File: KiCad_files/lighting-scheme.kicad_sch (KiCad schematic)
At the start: 11 parts, among them J1 Conn_01x03

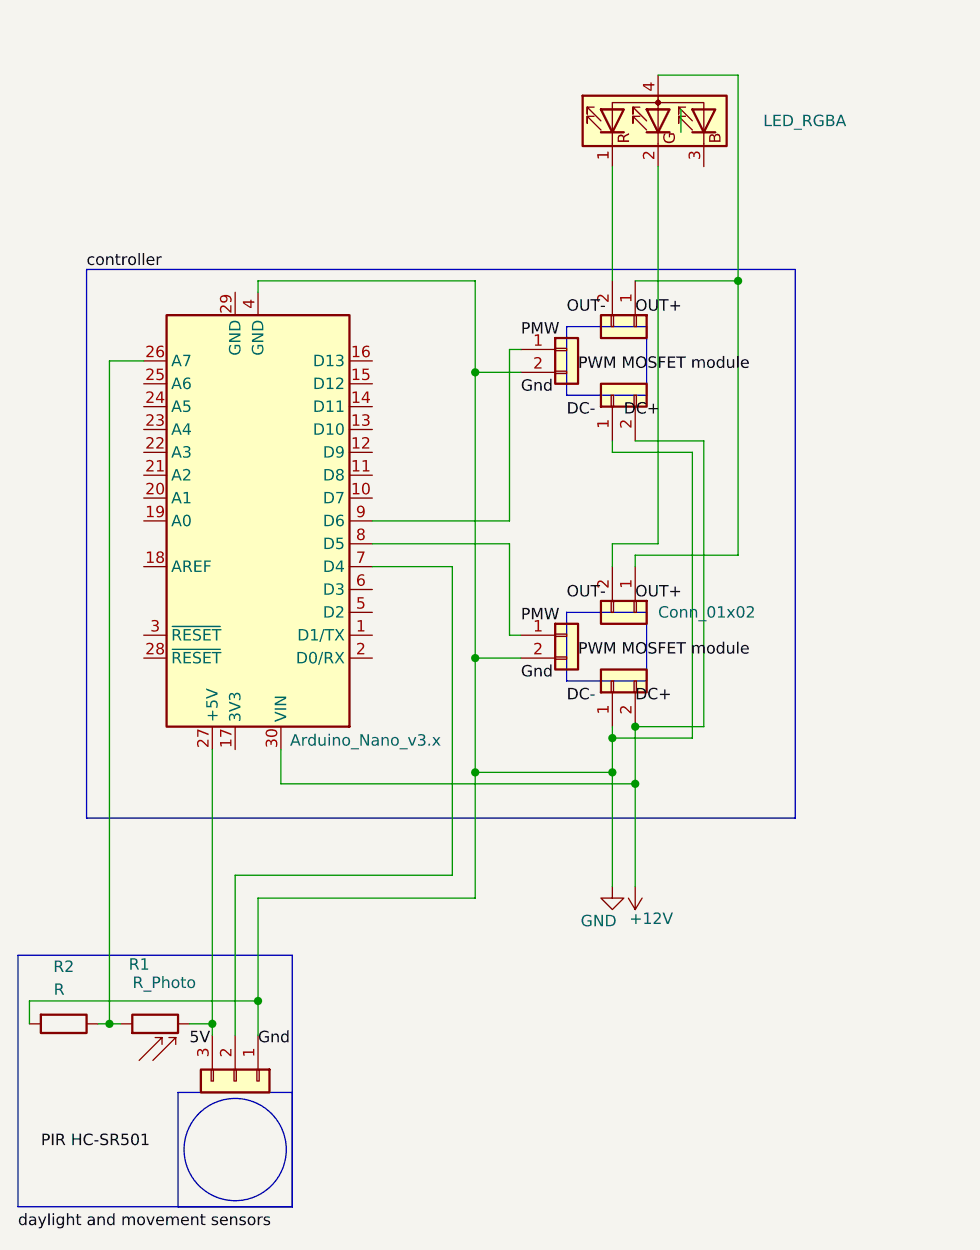
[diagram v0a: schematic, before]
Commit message: aktuallizacja folder z kicad 2
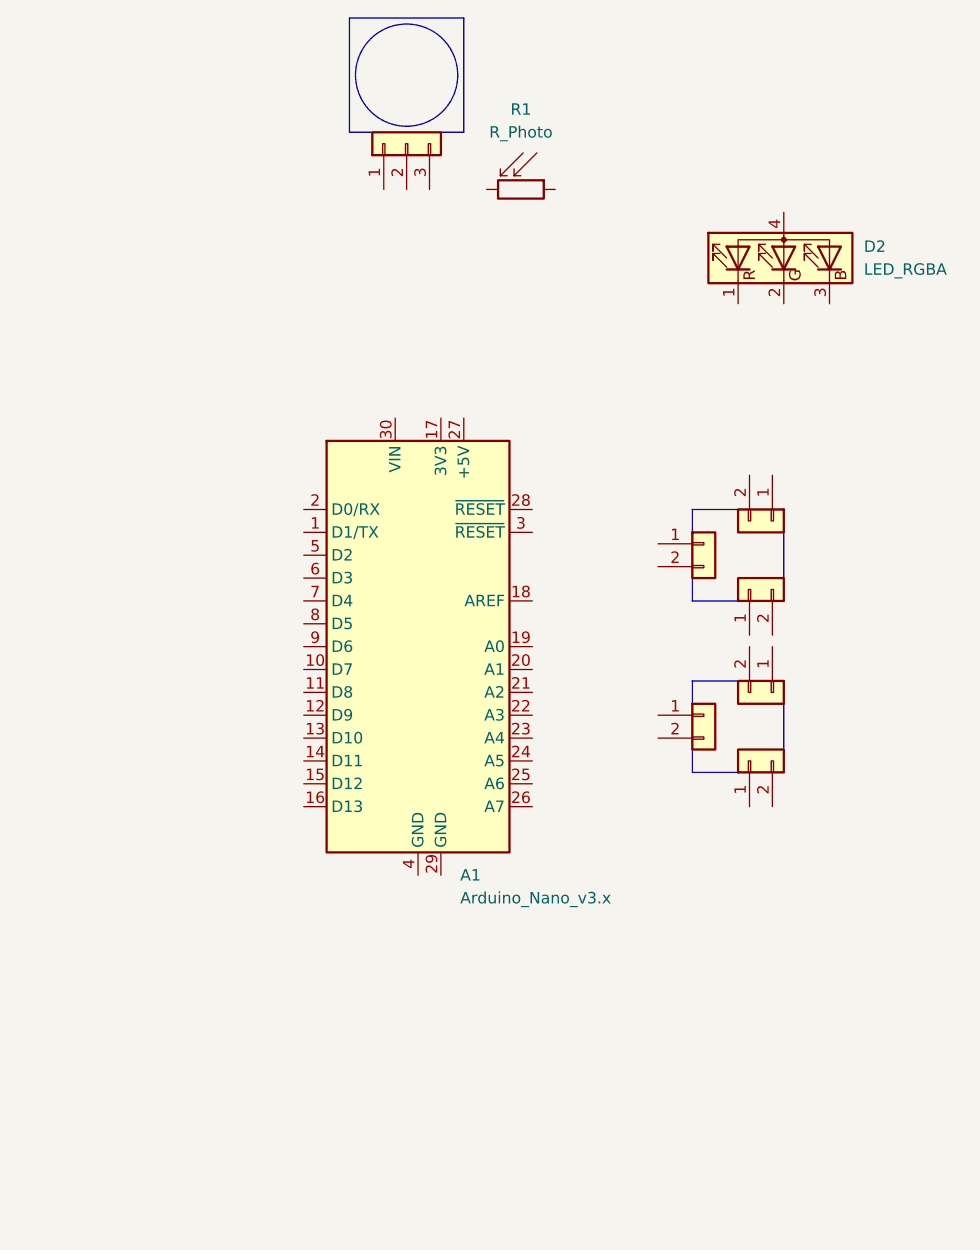
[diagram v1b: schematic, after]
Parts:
- removed R2: R, symbol Device:R
- MOSFET_CTRL2: value Conn_01x02 -> ~
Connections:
- net at MOSFET_CTRL2.2 (Pin_2): no longer D2.2 (GK)
- net at MOSFET_CTRL3.1 (Pin_1): no longer A1.9 (D6)
- net at MOSFET_CTRL.1 (Pin_1): no longer A1.8 (D5)
- net at A1.26 (A7): no longer R1.1
- net at A1.7 (D4): no longer J1.2 (Pin_2)
- net at D2.1 (RK): no longer MOSFET_CTRL5.2 (Pin_2)
- removed net +12V: A1.30 (VIN), MOSFET_CTRL1.2 (Pin_2), MOSFET_CTRL4.2 (Pin_2)
- removed net GND: A1.4 (GND), J1.1 (Pin_1), MOSFET_CTRL.2 (Pin_2), MOSFET_CTRL1.1 (Pin_1), MOSFET_CTRL3.2 (Pin_2), MOSFET_CTRL4.1 (Pin_1)
- now unconnected: A1.27 (+5V), D2.4 (A), J1.3 (Pin_3), MOSFET_CTRL2.1 (Pin_1), MOSFET_CTRL5.1 (Pin_1), R1.2
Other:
- moved on the sheet: R1
